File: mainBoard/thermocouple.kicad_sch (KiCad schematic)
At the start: 54 parts, among them J16 4DB-P108-02, J3 4DB-P108-02, J5 4DB-P108-02, U10 OPA333AIDCKT, U11 DS18B20+, U5 DS18B20+, U6 OPA333AIDCKT, U8 OPA333AIDCKT, U9 DS18B20+

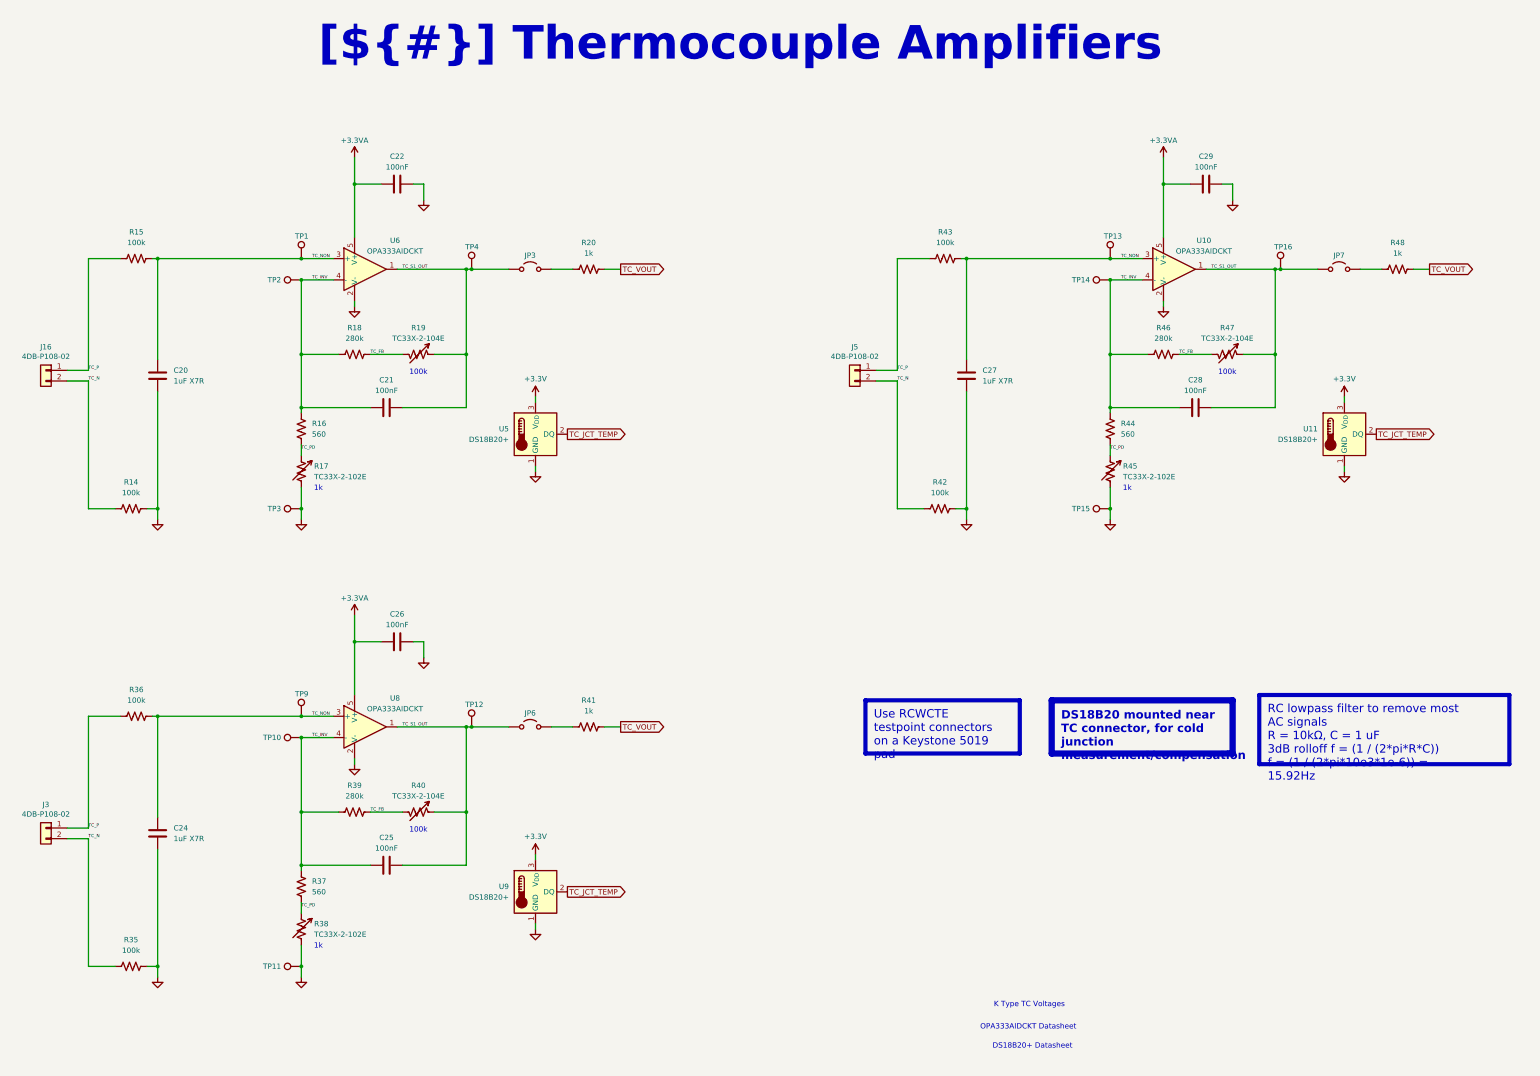
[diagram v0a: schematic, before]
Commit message: working on pcb layout after bringing in work from laptop
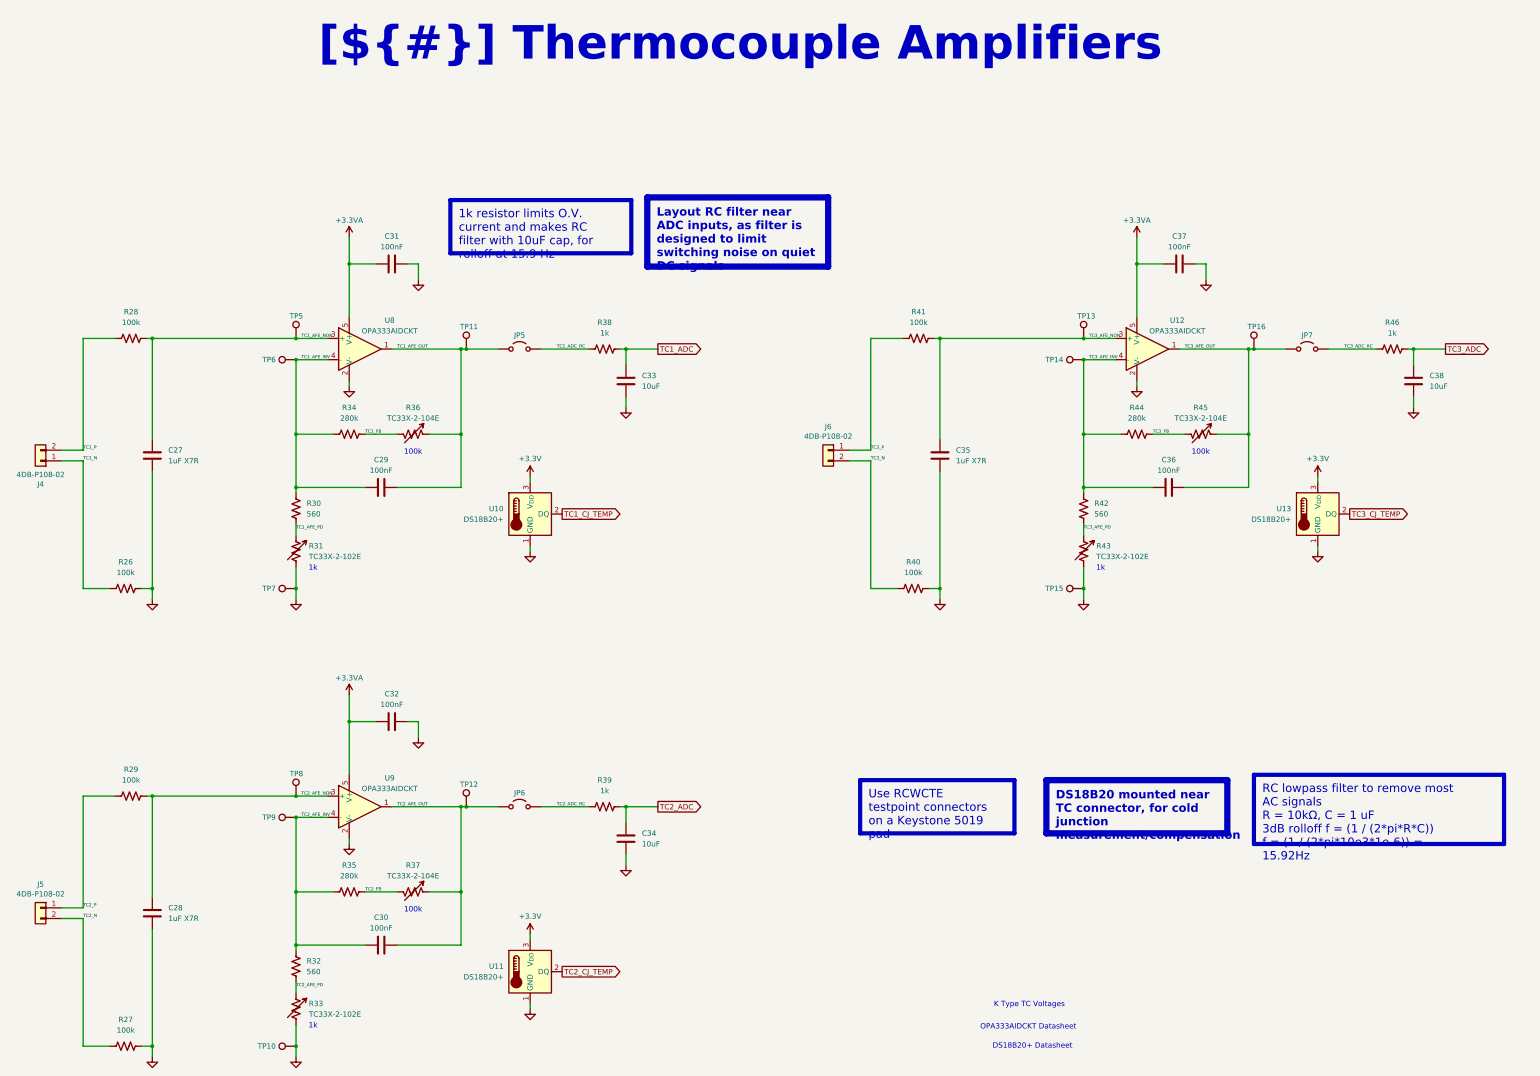
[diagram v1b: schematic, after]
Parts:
- removed C24, C27: 1uF X7R, Capacitor_SMD:C_0603_1608Metric_Pad1.08x0.95mm_HandSolder, symbol Device:C
- removed C25, C26, C29: 100nF, Capacitor_SMD:C_0805_2012Metric_Pad1.18x1.45mm_HandSolder, symbol Device:C
- removed J3: 4DB-P108-02, 4DB_P108_02:CONN_4DB-P108-02_TEC, symbol Connector_Generic:Conn_01x02
- removed R36, R43: 100k, Resistor_SMD:R_0603_1608Metric_Pad0.98x0.95mm_HandSolder, symbol Device:R_US
- removed R37: 560, Resistor_SMD:R_0603_1608Metric_Pad0.98x0.95mm_HandSolder, symbol Device:R_US
- removed R38: TC33X-2-102E, Potentiometer_SMD:Potentiometer_Bourns_TC33X_Vertical, symbol Device:R_Variable_US
- removed R40, R47: TC33X-2-104E, Potentiometer_SMD:Potentiometer_Bourns_TC33X_Vertical, symbol Device:R_Variable_US
- removed R48: 1k, Resistor_SMD:R_0603_1608Metric_Pad0.98x0.95mm_HandSolder, symbol Device:R_US
- removed TP11: TestPoint, TestPoint:TestPoint_Keystone_5019_Miniature, symbol Connector:TestPoint
- removed U10, U8: OPA333AIDCKT, Package_SO:SOIC-8_3.9x4.9mm_P1.27mm, symbol Amplifier_Operational:OPA333xxDBV
- removed U9: DS18B20+, Package_TO_SOT_THT:TO-92_Inline, symbol Sensor_Temperature:DS18B20
- added C30, C32, C36, C37: 100nF, Capacitor_SMD:C_0805_2012Metric_Pad1.18x1.45mm_HandSolder, symbol Device:C
- added C33, C34, C38: 10uF, Capacitor_SMD:C_0603_1608Metric_Pad1.08x0.95mm_HandSolder, symbol Device:C
- added C35: 1uF X7R, Capacitor_SMD:C_0603_1608Metric_Pad1.08x0.95mm_HandSolder, symbol Device:C
- added J6: 4DB-P108-02, 4DB_P108_02:CONN_4DB-P108-02_TEC, symbol Connector_Generic:Conn_01x02
- added R27, R29, R40: 100k, Resistor_SMD:R_0603_1608Metric_Pad0.98x0.95mm_HandSolder, symbol Device:R_US
- added R32: 560, Resistor_SMD:R_0603_1608Metric_Pad0.98x0.95mm_HandSolder, symbol Device:R_US
- added R33, R43: TC33X-2-102E, Potentiometer_SMD:Potentiometer_Bourns_TC33X_Vertical, symbol Device:R_Variable_US
- added R37: TC33X-2-104E, Potentiometer_SMD:Potentiometer_Bourns_TC33X_Vertical, symbol Device:R_Variable_US
- added TP8: TestPoint, TestPoint:TestPoint_Keystone_5019_Miniature, symbol Connector:TestPoint
- added U12, U9: OPA333AIDCKT, Package_SO:SOIC-8_3.9x4.9mm_P1.27mm, symbol Amplifier_Operational:OPA333xxDBV
- added U13: DS18B20+, Package_TO_SOT_THT:TO-92_Inline, symbol Sensor_Temperature:DS18B20
- C28: value 100nF -> 1uF X7R; footprint Capacitor_SMD:C_0805_2012Metric_Pad1.18x1.45mm_HandSolder -> Capacitor_SMD:C_0603_1608Metric_Pad1.08x0.95mm_HandSolder
- R35: value 100k -> 280k
- R39, R46: value 280k -> 1k
- R41: value 1k -> 100k
- R42: value 100k -> 560
- R44: value 560 -> 280k
- R45: value TC33X-2-102E -> TC33X-2-104E
- renumbered C20 to C27, C21 to C29, C22 to C31, J16 to J4, JP3 to JP5, R14 to R26, R15 to R28, R16 to R30, R17 to R31, R18 to R34, R19 to R36, R20 to R38, TP4 to TP11, TP1 to TP5, TP2 to TP6, TP3 to TP7, U5 to U10, U6 to U8
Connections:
- net +3.3V: now also U13.3 (V_{DD})
- net +3.3VA: now also C32.1, C37.1, U12.5 (V+), U9.5 (V+)
- net GND: now also C28.2, TP10.1, C32.2, C33.2, C34.2, C35.2, C37.2, C38.2, R27.2, R33.2, R40.2, R43.2, U12.2 (V-), U13.1 (GND), U9.2 (V-); no longer R35.2, R42.2, R45.2
- net TC3_ADC_RC: now reaches JP7.2 (B)
- net TC3_ADC_RC: now also R46.1
- net TC1_ADC_RC: now reaches JP5.2 (B), R38.1
- net TC2_ADC_RC: now reaches JP6.2 (B)
- net TC2_ADC_RC: now also R39.1; no longer R41.1
- net TC_FB renamed TC1_FB
- net TC1_FB: no longer R39.2, R46.2
- removed net TC_INV: C28.1, C29.1, R30.1, R34.1, R39.1, R44.1, R46.1, TP10.1, TP14.1, TP6.1, U8.4 (-)
- net TC_JCT_TEMP renamed TC1_CJ_TEMP
- net TC1_CJ_TEMP: no longer U11.2 (DQ)
- removed net TC_N: J4.2 (Pin_2), J5.2 (Pin_2), R26.1, R35.1, R42.1
- net TC_NON renamed TC1_AFE_NON
- net TC1_AFE_NON: no longer TP13.1, TP9.1
- removed net TC_P: J4.1 (Pin_1), J5.1 (Pin_1), R28.1
- net TC_PD renamed TC1_AFE_PD
- net TC1_AFE_PD: no longer R44.2, R45.1
- net TC_S1_OUT renamed TC1_AFE_OUT
- net TC1_AFE_OUT: no longer C28.2, JP6.1 (A), JP7.1 (A), TP12.1, TP16.1
- net TC_VOUT renamed TC1_ADC
- net TC1_ADC: now also C33.1; no longer R41.2
- new net TC1_AFE_INV: C29.1, R30.1, R34.1, TP6.1, U8.4 (-)
- new net TC1_N: J4.1 (Pin_1), R26.1
- new net TC1_P: J4.2 (Pin_2), R28.1
- new net TC2_ADC: C34.1, R39.2
- new net TC2_AFE_INV: C30.1, R32.1, R35.1, TP9.1, U9.4 (-)
- new net TC2_AFE_NON: C28.1, R29.2, TP8.1, U9.3 (+)
- new net TC2_AFE_OUT: C30.2, JP6.1 (A), R37.1, TP12.1, U9.1
- new net TC2_AFE_PD: R32.2, R33.1
- new net TC2_CJ_TEMP: U11.2 (DQ)
- new net TC2_FB: R35.2, R37.2
- new net TC2_N: J5.2 (Pin_2), R27.1
- new net TC2_P: J5.1 (Pin_1), R29.1
- new net TC3_ADC: C38.1, R46.2
- new net TC3_AFE_INV: C36.1, R42.1, R44.1, TP14.1, U12.4 (-)
- new net TC3_AFE_NON: C35.1, R41.2, TP13.1, U12.3 (+)
- new net TC3_AFE_OUT: C36.2, JP7.1 (A), R45.1, TP16.1, U12.1
- new net TC3_AFE_PD: R42.2, R43.1
- new net TC3_CJ_TEMP: U13.2 (DQ)
- new net TC3_FB: R44.2, R45.2
- new net TC3_N: J6.2 (Pin_2), R40.1
- new net TC3_P: J6.1 (Pin_1), R41.1
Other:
- moved on the sheet: C27, C29, C31, J4, JP5, R26, R28, R30, R31, R34, R36, R38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
